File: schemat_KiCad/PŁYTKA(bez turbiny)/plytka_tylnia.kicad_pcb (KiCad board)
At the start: 2 copper layers, 200 x 150 mm, 80 parts, among them J1 CONN_01X04, J2 CONN_01X04, J3 CONN_01X04, J4 CONN_01X04, J5 CONN_01X04, J6 CONN_01X04, J7 PIN10, J8 CONN_01X04, J9 CONN_01X04, P1 USB_OTG, T1 KTIR0711S, T2 KTIR0711S, T3 KTIR0711S, T4 KTIR0711S, T5 KTIR0711S, T6 KTIR0711S, T7 KTIR0711S, T8 KTIR0711S, U1 AS5048A, U2 AS5048A

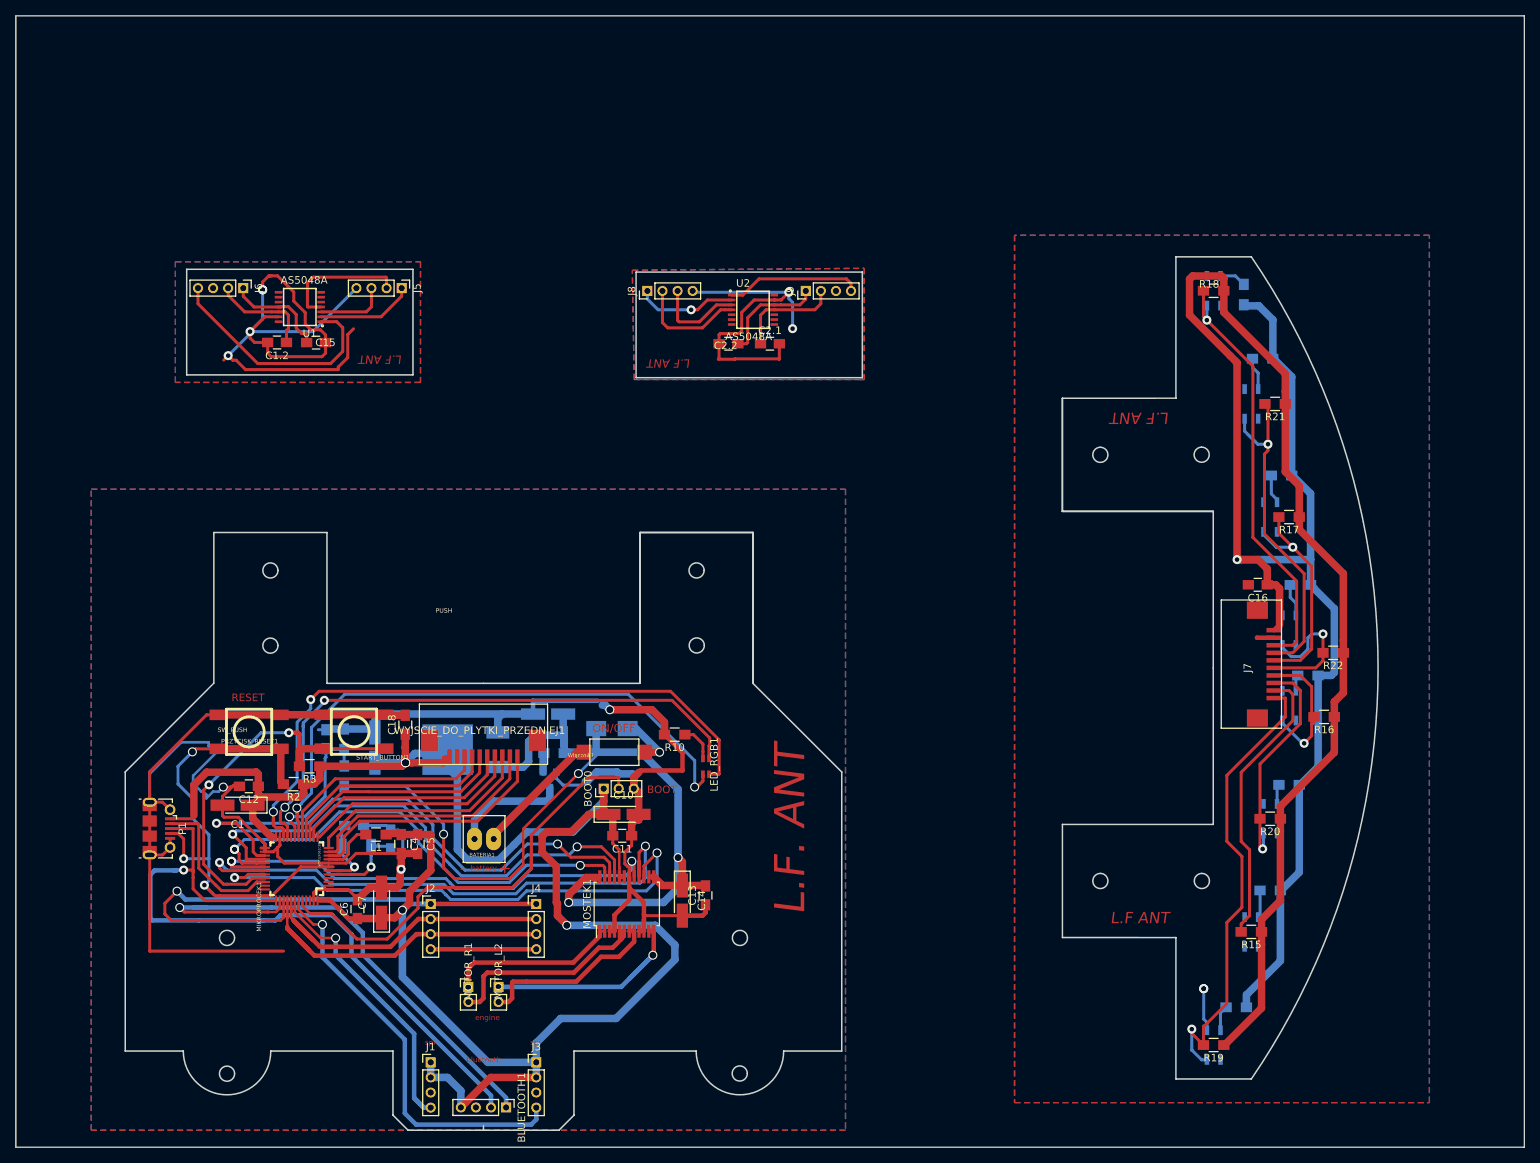
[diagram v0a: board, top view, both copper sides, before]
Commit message: poprawiona, odchudzona, zaokraglona
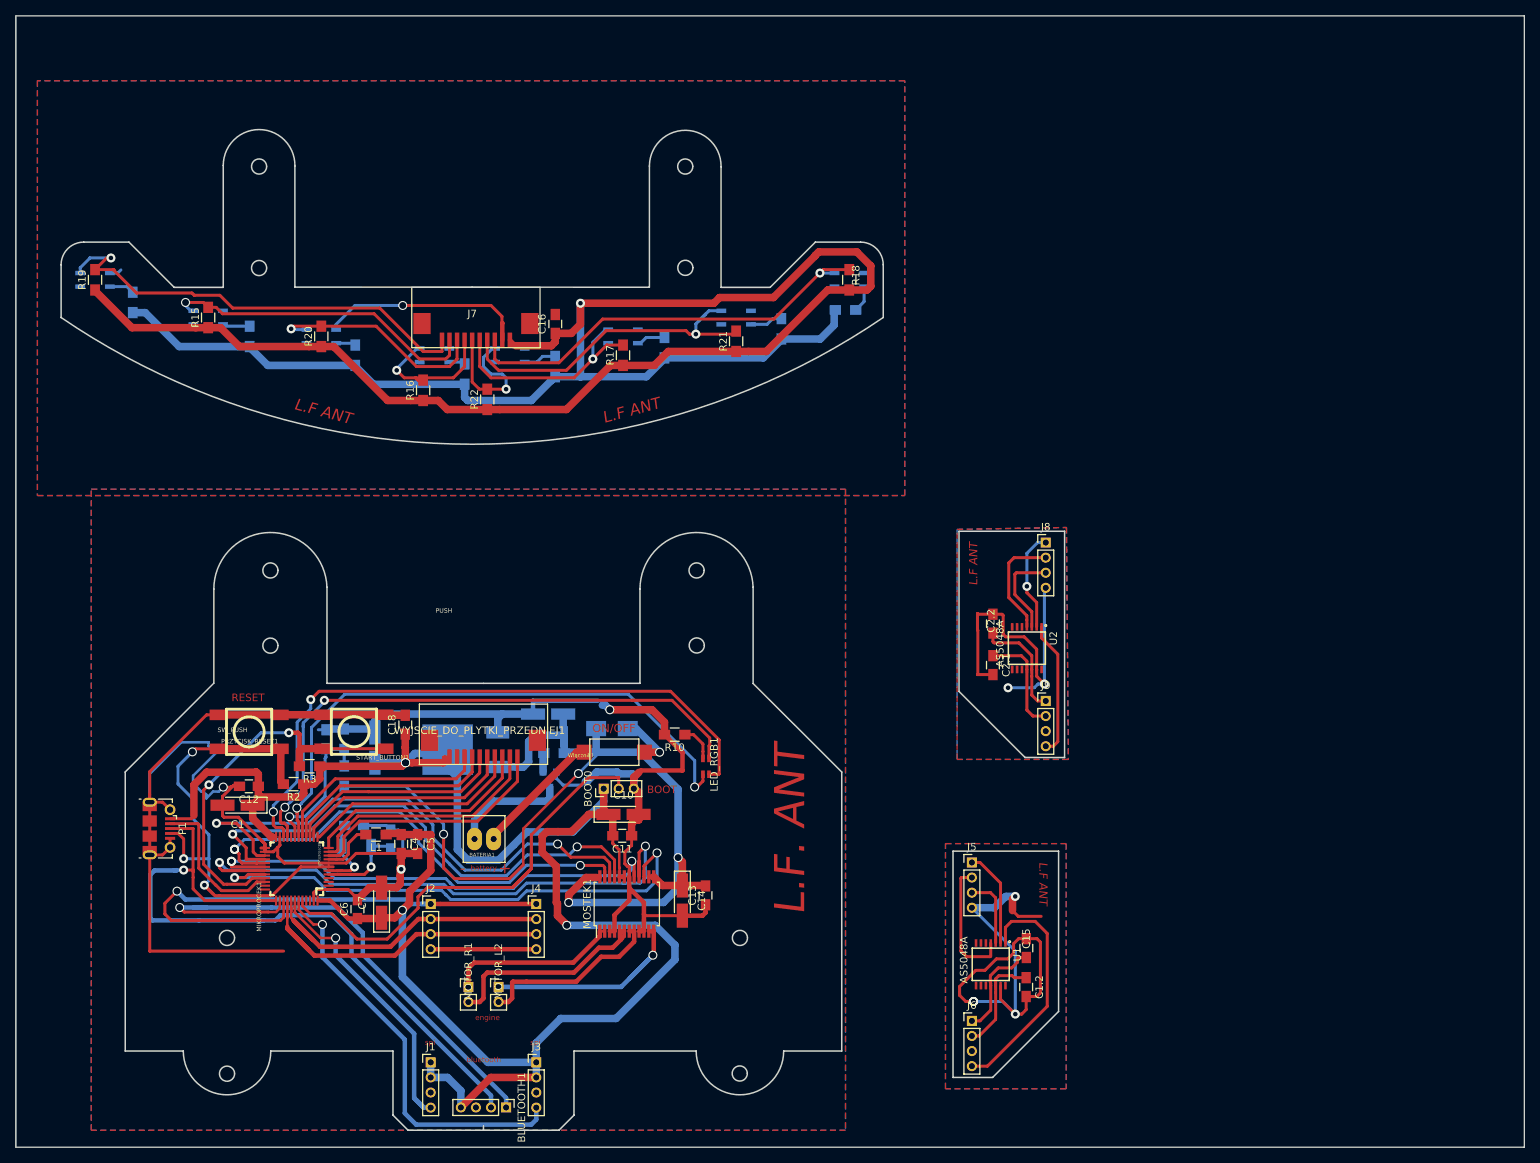
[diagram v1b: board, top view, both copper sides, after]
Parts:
- moved R19 179.7 mm to (45.5, 65.0), turned to 90 degrees
- moved T5 179.7 mm to (45.5, 65.0), turned to 90 degrees
- moved R11 173.6 mm to (50.5, 68.0), turned to 90 degrees
- moved R15 160.5 mm to (60.5, 70.0), turned to 90 degrees
- moved T1 160.5 mm to (60.5, 70.0), turned to 90 degrees
- moved R1 154.0 mm to (66.0, 72.5), turned to 90 degrees
- moved R20 141.1 mm to (75.5, 72.5), turned to 90 degrees
- moved T6 141.1 mm to (75.5, 72.5), turned to 90 degrees
- moved J6 137.0 mm to (161.8, 163.2), turned to 0 degrees
- moved R12 136.3 mm to (80.0, 75.0), turned to 90 degrees
- moved C1.2 131.0 mm to (169.0, 158.8), turned to 270 degrees
- moved R16 127.1 mm to (89.0, 79.6), turned to 90 degrees
- moved U1 126.4 mm to (164.3, 155.7), turned to 270 degrees
- moved C15 123.7 mm to (169.0, 153.6), turned to 90 degrees
- moved T2 122.5 mm to (90.5, 75.0), turned to 90 degrees
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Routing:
- net GND: track 333.4 -> 356.9 mm, vias 5 -> 4
- net /GND1: track 84.5 -> 70.2 mm
- net /T2: track 70.0 -> 74.1 mm, vias 0 -> 1
- net /T1: track 95.3 -> 93.6 mm
- net VCC: track 569.1 -> 570.7 mm
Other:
- outline, holes or cut-outs redrawn
